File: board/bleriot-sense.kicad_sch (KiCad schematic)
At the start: 25 parts, among them J1 POWER, J2 INPUT, U1 LM1117MP-3.3, U2 PAN2110P0AA, U3 PY32F030F1xPx, X1 SWD, Y1 16MHz

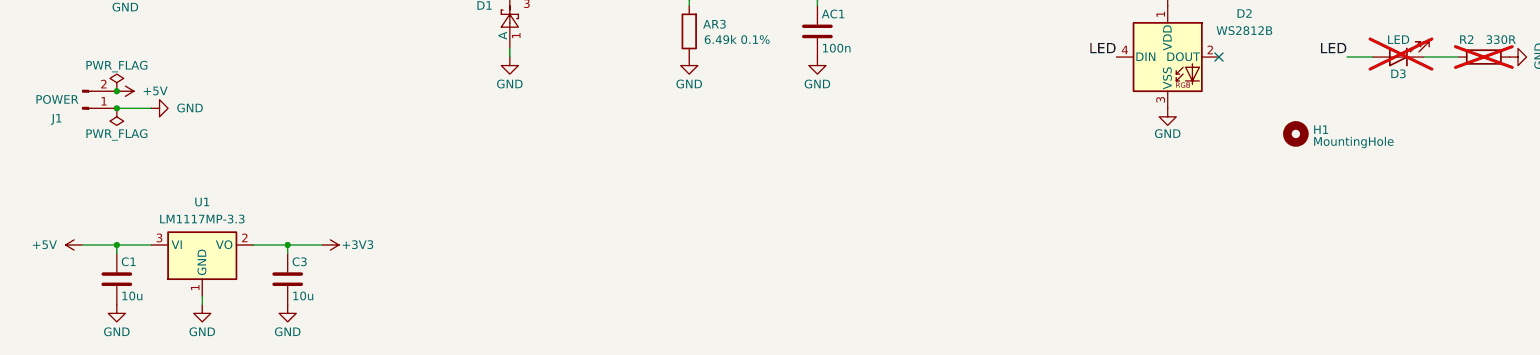
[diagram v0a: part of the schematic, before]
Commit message: WIP
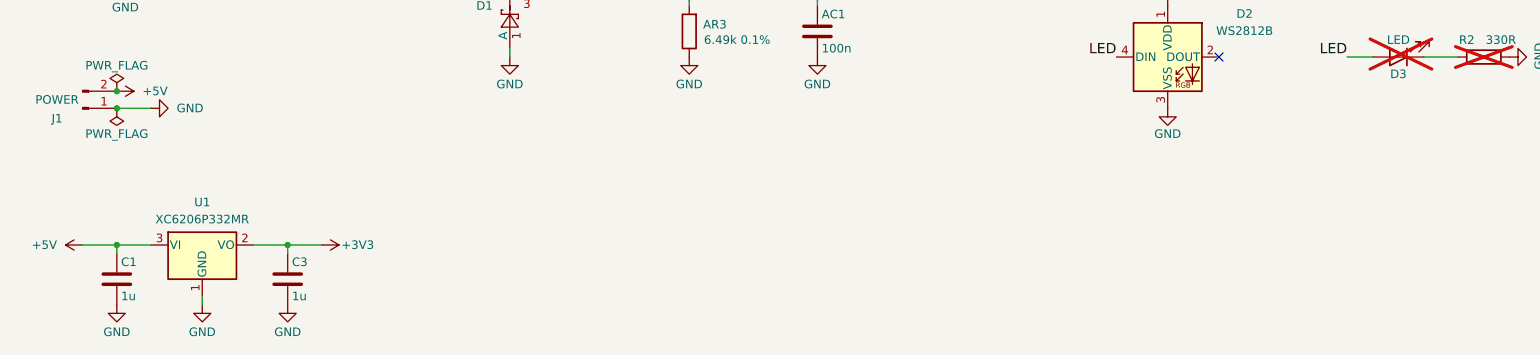
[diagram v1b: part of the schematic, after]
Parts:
- removed H1: MountingHole, MountingHole:MountingHole_3.7mm_Pad_Via, symbol Mechanical:MountingHole
- removed U1: LM1117MP-3.3, Package_TO_SOT_SMD:SOT-223-3_TabPin2, symbol Regulator_Linear:LM1117MP-3.3
- added U1: XC6206P332MR, Package_TO_SOT_SMD:SOT-23-3, symbol Regulator_Linear:XC6206PxxxMR
- C1, C3: value 10u -> 1u
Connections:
- net +3V3: now also U1.2 (VO)
- net +5V: now also U1.3 (VI)
- net GND: now also U1.1 (GND)
